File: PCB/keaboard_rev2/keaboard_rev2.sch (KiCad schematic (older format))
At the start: 80 parts, among them K01 KEYSW, K02 KEYSW, K03 KEYSW, K04 KEYSW, K05 KEYSW, K06 KEYSW, K07 KEYSW, K08 KEYSW, K09 KEYSW, K10 KEYSW, K11 KEYSW, K12 KEYSW, K13 KEYSW, K14 KEYSW, K15 KEYSW, K16 KEYSW, K17 KEYSW, K18 KEYSW, K19 KEYSW, K20 KEYSW, K21 KEYSW, K22 KEYSW, K23 KEYSW, K24 KEYSW, K25 KEYSW, U1 ProMicro

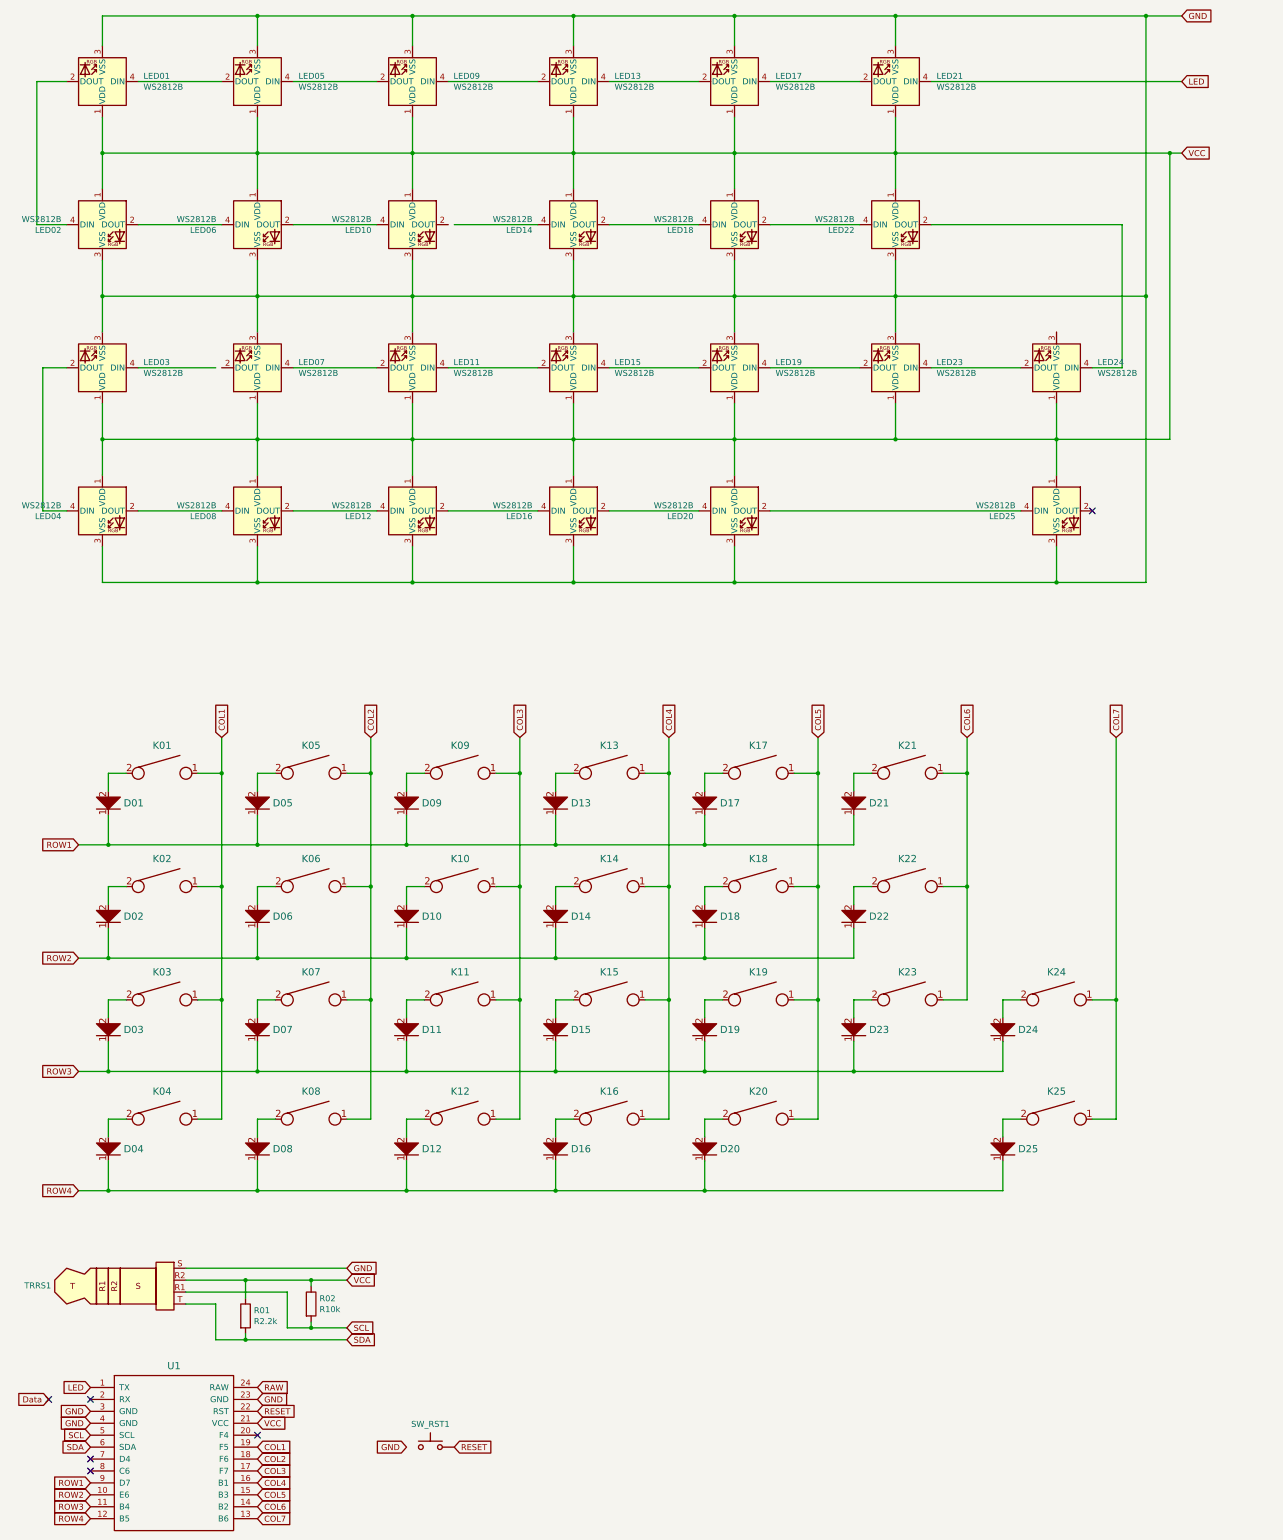
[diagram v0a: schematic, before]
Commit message: WIP rev2
Just traces remaining
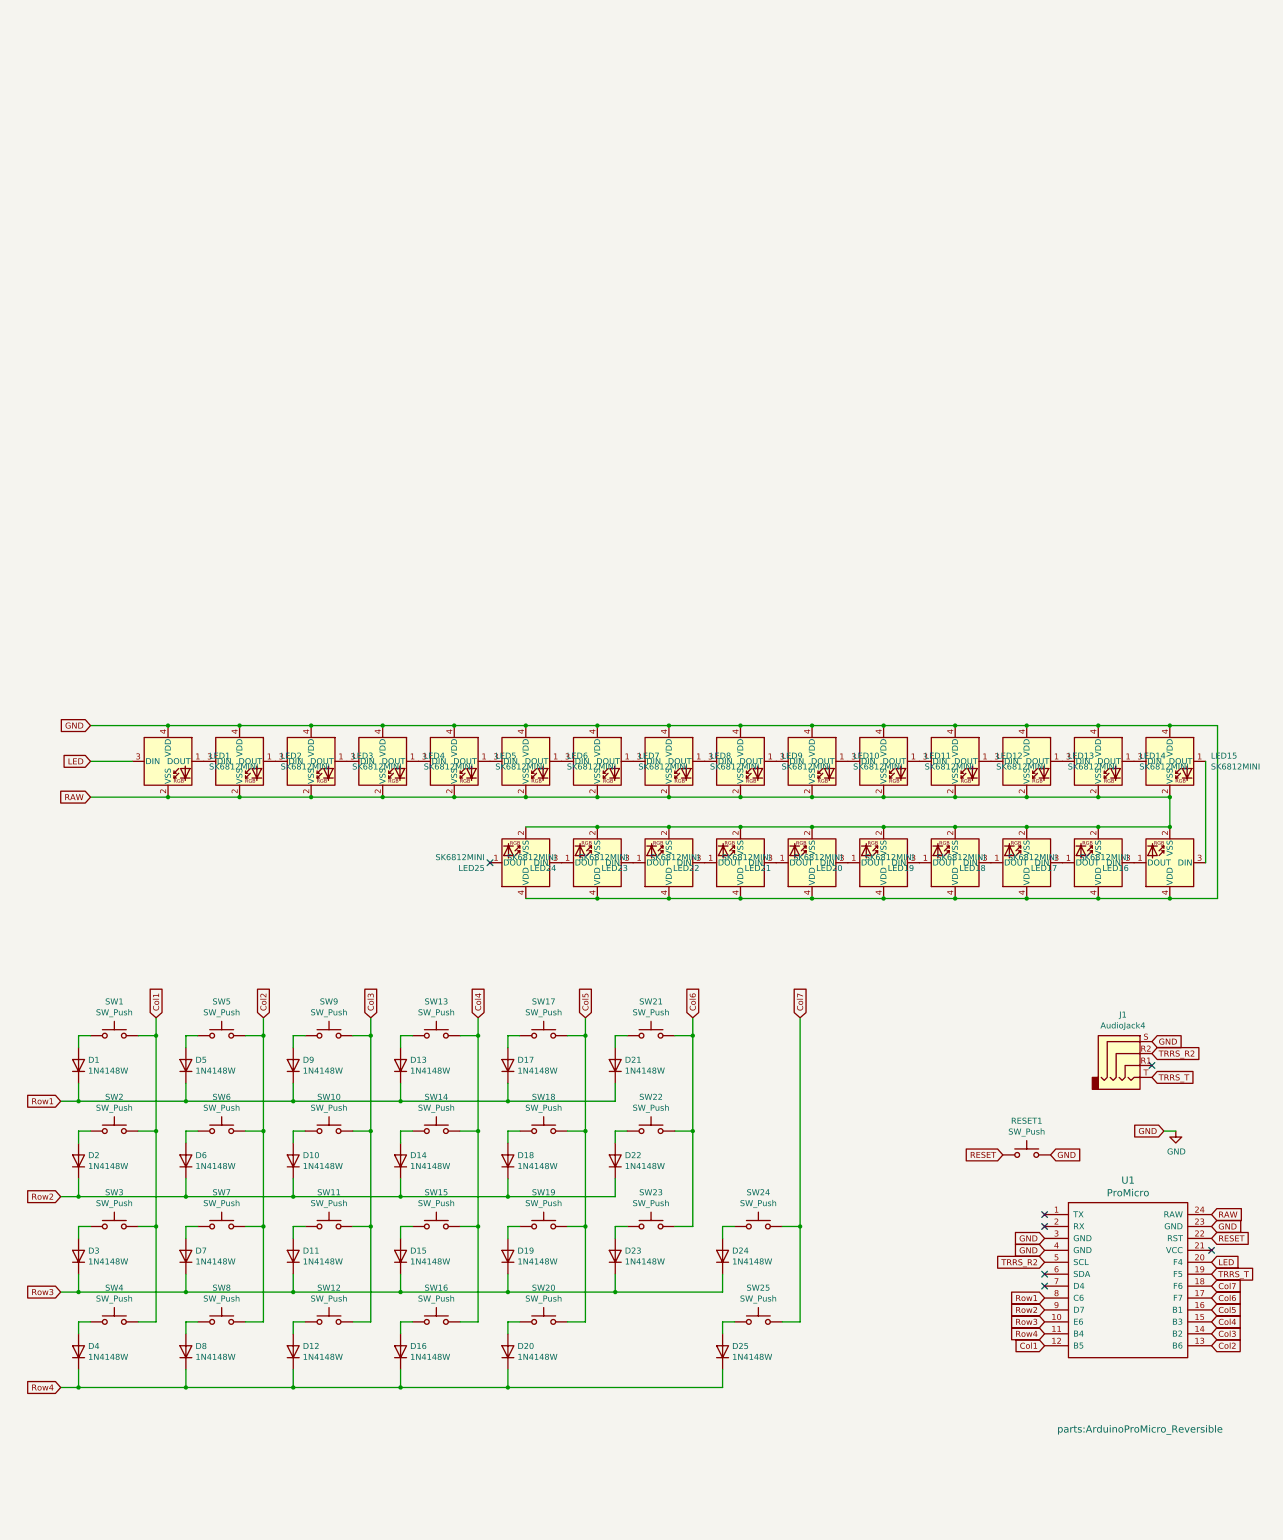
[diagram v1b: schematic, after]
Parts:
- removed D01, D02, D03, D04, D05, D06, D07, D08, D09, D10, D11, D12, D13, D14, D15, D16, D17, D18, D19, D20, D21, D22, D23, D24, D25: D, parts:D_SOD123_reversible, symbol keyboard_parts:D
- removed K01, K02, K03, K04, K05, K06, K07, K08, K09, K10, K11, K12, K13, K14, K15, K16, K17, K18, K19, K20, K21, K22, K23, K24, K25: KEYSW, parts:Kailh_socket_MX_reversible, symbol keyboard_parts:KEYSW
- removed LED01, LED02, LED03, LED04, LED05, LED06, LED07, LED08, LED09, LED10, LED11, LED12, LED13, LED14, LED15, LED16, LED17, LED18, LED19, LED20, LED21, LED22, LED23, LED24, LED25: WS2812B, LED_SMD:LED_WS2812B_PLCC4_5.0x5.0mm_P3.2mm, symbol LED:WS2812B
- removed R01: R2.2k, symbol Device:R
- removed R02: R10k, symbol Device:R
- removed SW_RST1: SW_EVQ-9P701P, parts:SW_EVQ-9P701P_reversible, symbol Switch:SW_MEC_5G
- removed TRRS1: TRRS Jack, parts:TRRS-PJ-320A_reversible, symbol keaboard_rev2-rescue:AudioPlug4-Connector-keaboard_rev1-rescue
- added D1, D10, D11, D12, D13, D14, D15, D16, D17, D18, D19, D2, D20, D21, D22, D23, D24, D25, D3, D4, D5, D6, D7, D8, D9: 1N4148W, parts:D_SOD123_reversible, symbol Diode:1N4148W
- added J1: AudioJack4, parts:TRRS-PJ-320A_reversible, symbol Connector:AudioJack4
- added LED1, LED10, LED11, LED12, LED13, LED14, LED15, LED16, LED17, LED18, LED19, LED2, LED20, LED21, LED22, LED23, LED24, LED25, LED3, LED4, LED5, LED6, LED7, LED8, LED9: SK6812MINI, parts:YS-SK6812MINI-E_reversible, symbol LED:SK6812MINI
- added RESET1: SW_Push, parts:SW_EVQ-9P701P_reversible, symbol Switch:SW_Push
- added SW1, SW10, SW11, SW12, SW13, SW14, SW15, SW16, SW17, SW18, SW19, SW2, SW20, SW21, SW22, SW23, SW24, SW25, SW3, SW4, SW5, SW6, SW7, SW8, SW9: SW_Push, keyswitches:Kailh_socket_PG1350_reversible, symbol Switch:SW_Push
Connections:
- net GND: now also J1.S, LED1.4 (VDD), LED10.4 (VDD), LED11.4 (VDD), LED12.4 (VDD), LED13.4 (VDD), LED14.4 (VDD), LED15.4 (VDD), LED16.4 (VDD), LED17.4 (VDD), LED18.4 (VDD), LED19.4 (VDD), LED2.4 (VDD), LED20.4 (VDD), LED21.4 (VDD), LED22.4 (VDD), LED23.4 (VDD), LED24.4 (VDD), LED25.4 (VDD), LED3.4 (VDD), LED4.4 (VDD), LED5.4 (VDD), LED6.4 (VDD), LED7.4 (VDD), LED8.4 (VDD), LED9.4 (VDD), RESET1.2
- net LED: now also U1.20 (F4), LED1.3 (DIN); no longer U1.1 (TX)
- net RAW: now also LED1.2 (VSS), LED10.2 (VSS), LED11.2 (VSS), LED12.2 (VSS), LED13.2 (VSS), LED14.2 (VSS), LED15.2 (VSS), LED16.2 (VSS), LED17.2 (VSS), LED18.2 (VSS), LED19.2 (VSS), LED2.2 (VSS), LED20.2 (VSS), LED21.2 (VSS), LED22.2 (VSS), LED23.2 (VSS), LED24.2 (VSS), LED25.2 (VSS), LED3.2 (VSS), LED4.2 (VSS), LED5.2 (VSS), LED6.2 (VSS), LED7.2 (VSS), LED8.2 (VSS), LED9.2 (VSS)
- net RESET: now also RESET1.1
- net Row1: now reaches U1.8 (C6)
- net Row1: now also D1.1 (K), D13.1 (K), D17.1 (K), D21.1 (K), D5.1 (K), D9.1 (K)
- net COL1 renamed TRRS_T
- net TRRS_T: now also J1.T
- net COL2 renamed Col7
- net Col7: now also SW24.2, SW25.2
- net COL3 renamed Col6
- net Col6: now also SW21.2, SW22.2, SW23.2
- net COL4 renamed Col5
- net Col5: now also SW17.2, SW18.2, SW19.2, SW20.2
- net COL5 renamed Col4
- net Col4: now also SW13.2, SW14.2, SW15.2, SW16.2
- net COL6 renamed Col3
- net Col3: now also SW10.2, SW11.2, SW12.2, SW9.2
- net COL7 renamed Col2
- net Col2: now also SW5.2, SW6.2, SW7.2, SW8.2
- net ROW1 renamed Row2
- net Row2: now also D10.1 (K), D14.1 (K), D18.1 (K), D2.1 (K), D22.1 (K), D6.1 (K)
- net ROW2 renamed Row3
- net Row3: now also D11.1 (K), D15.1 (K), D19.1 (K), D23.1 (K), D24.1 (K), D3.1 (K), D7.1 (K)
- net ROW3 renamed Row4
- net Row4: now also D12.1 (K), D16.1 (K), D20.1 (K), D25.1 (K), D4.1 (K), D8.1 (K)
- net ROW4 renamed Col1
- net Col1: now also SW1.2, SW2.2, SW3.2, SW4.2
- net SCL renamed TRRS_R2
- net TRRS_R2: now also J1.R2
- net SDA: no longer names the net of U1.6 (SDA)
- net VCC: no longer names the net of U1.21 (VCC)
- new net: LED1.1 (DOUT), LED2.3 (DIN)
- new net: D1.2 (A), SW1.1
- new net: D5.2 (A), SW5.1
- new net: D9.2 (A), SW9.1
- new net: D13.2 (A), SW13.1
- new net: D17.2 (A), SW17.1
- new net: D21.2 (A), SW21.1
- new net: D22.2 (A), SW22.1
- new net: D18.2 (A), SW18.1
- new net: D14.2 (A), SW14.1
- new net: D10.2 (A), SW10.1
- new net: D6.2 (A), SW6.1
- new net: D2.2 (A), SW2.1
- new net: D3.2 (A), SW3.1
- new net: D7.2 (A), SW7.1
- new net: D11.2 (A), SW11.1
- new net: D15.2 (A), SW15.1
- new net: D19.2 (A), SW19.1
- new net: D23.2 (A), SW23.1
- new net: D24.2 (A), SW24.1
- new net: D25.2 (A), SW25.1
- new net: D20.2 (A), SW20.1
- new net: D16.2 (A), SW16.1
- new net: D12.2 (A), SW12.1
- new net: D8.2 (A), SW8.1
- new net: D4.2 (A), SW4.1
- new net: LED2.1 (DOUT), LED3.3 (DIN)
- new net: LED3.1 (DOUT), LED4.3 (DIN)
- new net: LED4.1 (DOUT), LED5.3 (DIN)
- new net: LED5.1 (DOUT), LED6.3 (DIN)
- new net: LED6.1 (DOUT), LED7.3 (DIN)
- new net: LED7.1 (DOUT), LED8.3 (DIN)
- new net: LED8.1 (DOUT), LED9.3 (DIN)
- new net: LED10.3 (DIN), LED9.1 (DOUT)
- new net: LED10.1 (DOUT), LED11.3 (DIN)
- new net: LED11.1 (DOUT), LED12.3 (DIN)
- new net: LED12.1 (DOUT), LED13.3 (DIN)
- new net: LED13.1 (DOUT), LED14.3 (DIN)
- new net: LED14.1 (DOUT), LED15.3 (DIN)
- new net: LED15.1 (DOUT), LED16.3 (DIN)
- new net: LED16.1 (DOUT), LED17.3 (DIN)
- new net: LED17.1 (DOUT), LED18.3 (DIN)
- new net: LED18.1 (DOUT), LED19.3 (DIN)
- new net: LED19.1 (DOUT), LED20.3 (DIN)
- new net: LED20.1 (DOUT), LED21.3 (DIN)
- new net: LED21.1 (DOUT), LED22.3 (DIN)
- new net: LED22.1 (DOUT), LED23.3 (DIN)
- new net: LED23.1 (DOUT), LED24.3 (DIN)
- new net: LED24.1 (DOUT), LED25.3 (DIN)
- no-connect marks 6 -> 7
